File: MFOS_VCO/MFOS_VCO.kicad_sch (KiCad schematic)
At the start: 115 parts, among them J1 PWR, J10 Jack-DC, J11 Jack-DC, J12 Conn_01x01, J13 Conn_01x01, J14 Conn_01x01, J15 Conn_01x01, J16 Conn_01x01, J17 Conn_01x01, J18 Conn_01x01, J19 Conn_01x01, J2 Jack-DC, J21 Conn_01x01, J23 Conn_01x01, J25 Conn_01x01, J3 Jack-DC, J4 Jack-DC, J5 Jack-DC, J6 Jack-DC, J7 Jack-DC, J8 Jack-DC, J9 Jack-DC, Q1 PN4391, U1 OP275, U2 TL072, U3 SSM2212, U4 TL074, U5 LM13700, U6 TL072, U7 TL071

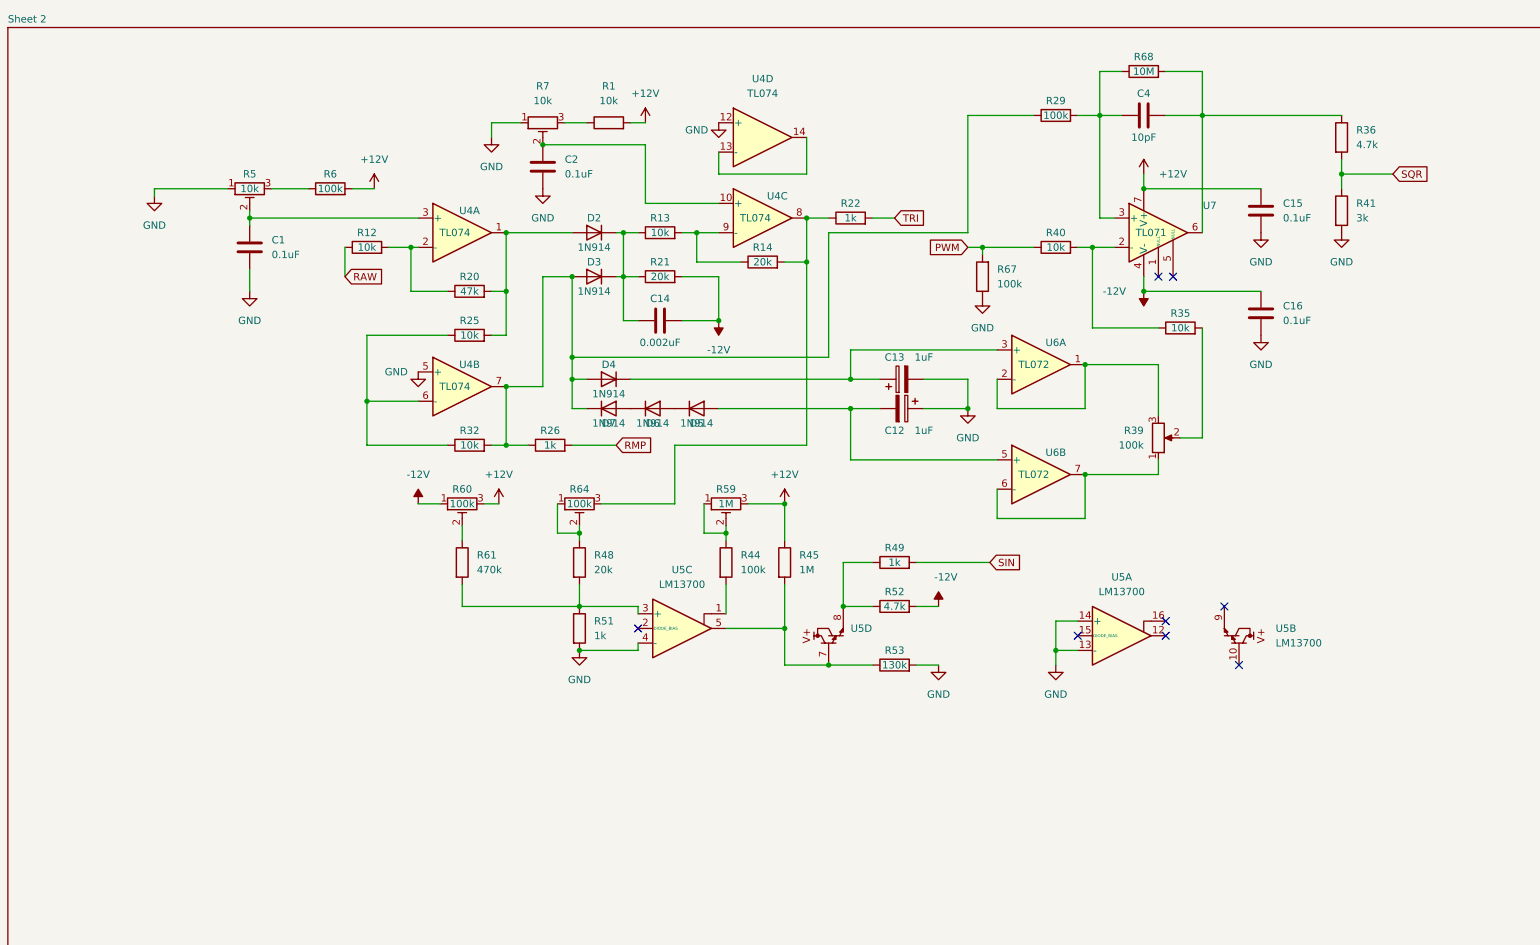
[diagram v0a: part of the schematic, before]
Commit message: yeah yeah
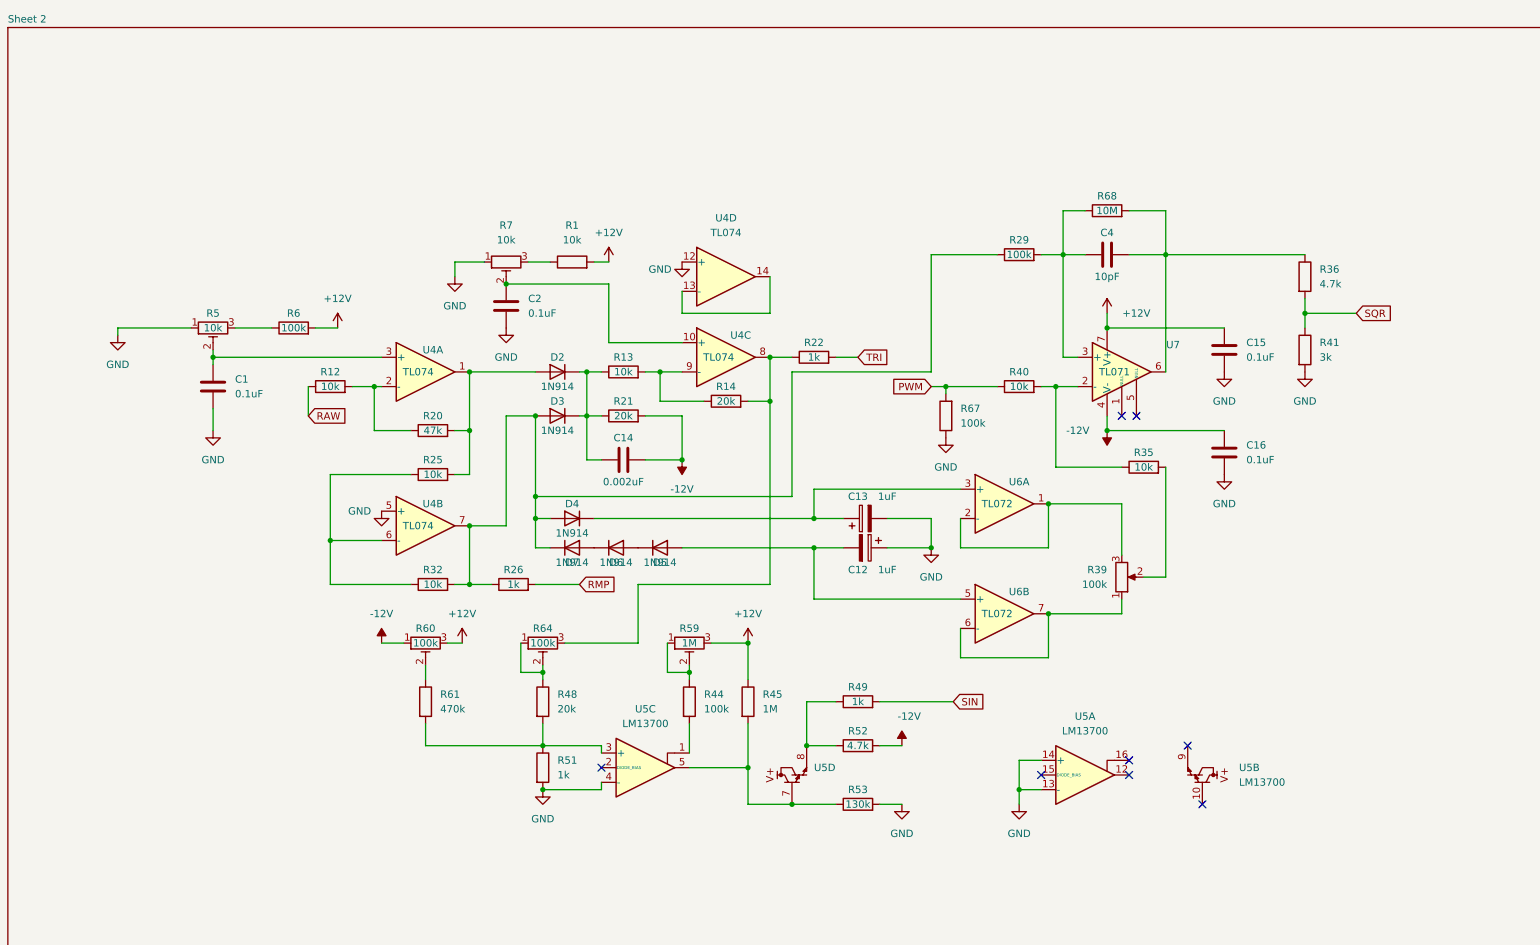
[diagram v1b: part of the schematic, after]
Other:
- moved on the sheet: C1, C12, C13, C14, C15, C16, C2, C4, D2, D3, D4, D5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
